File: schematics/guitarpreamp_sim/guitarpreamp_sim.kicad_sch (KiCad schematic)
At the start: 14 parts, among them U1 OPAMP, U2 OPAMP

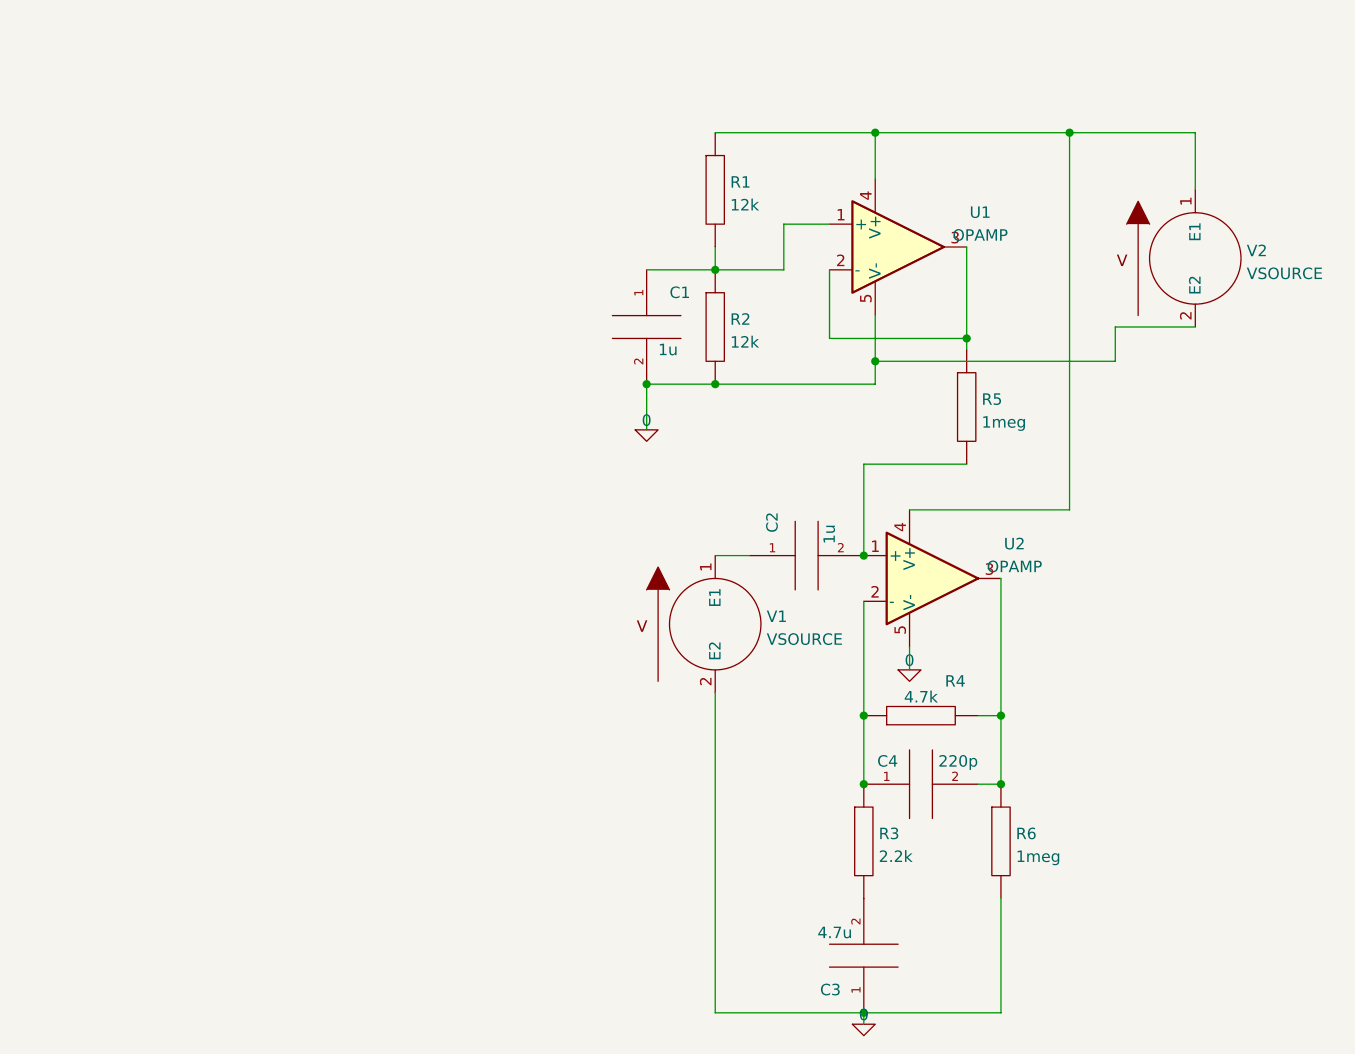
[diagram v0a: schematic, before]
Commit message: pcb: layout changes, c headers: documentation
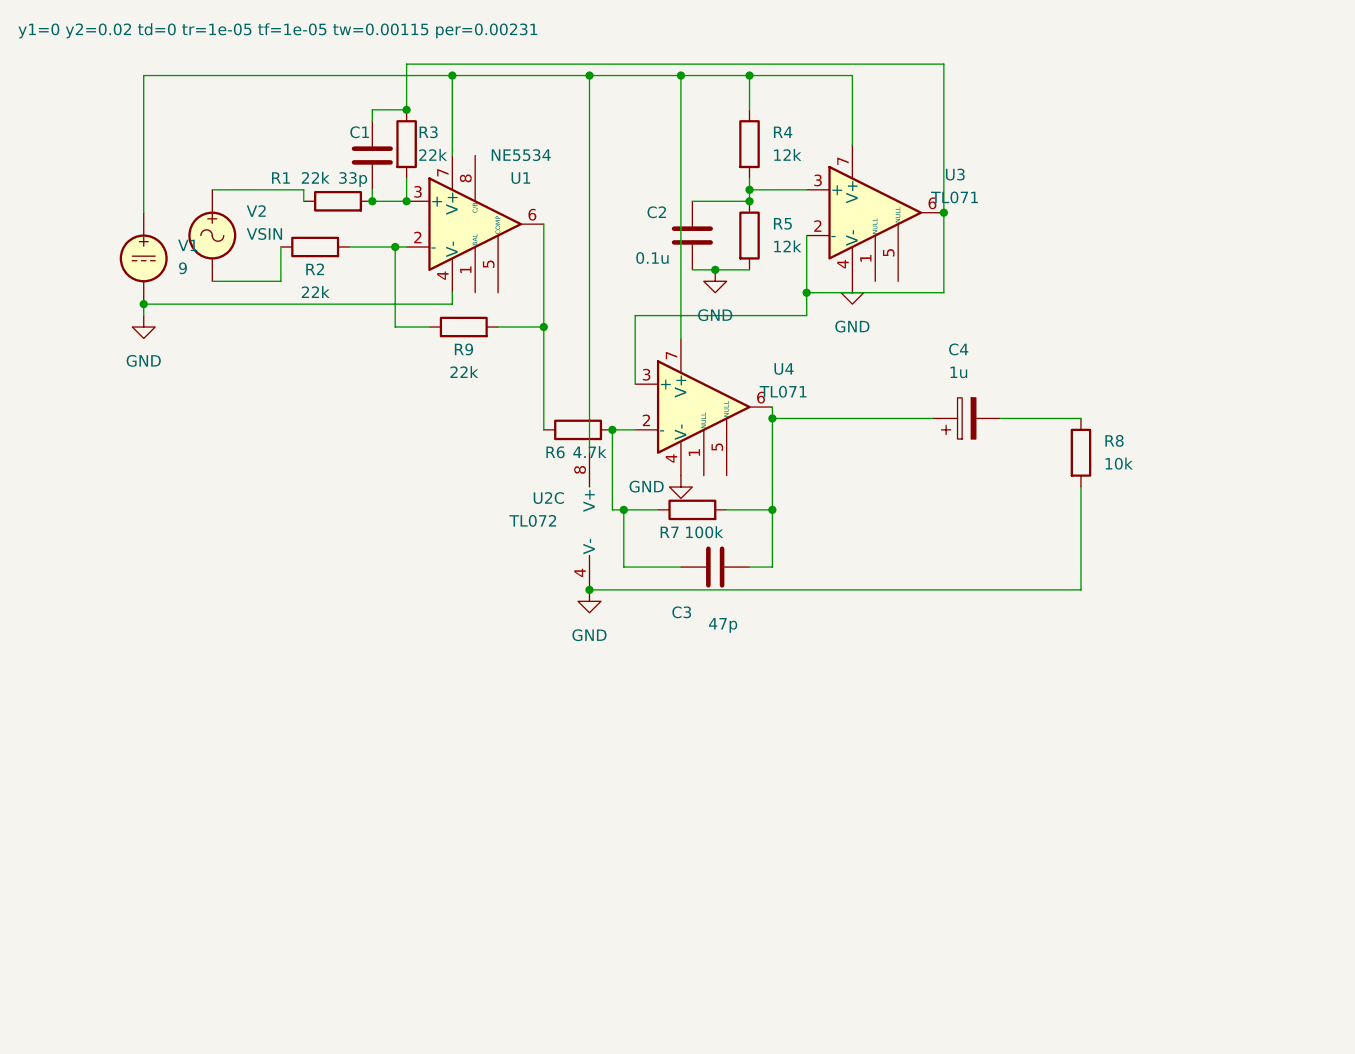
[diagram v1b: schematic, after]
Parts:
- removed C1, C2: 1u, symbol pspice:C
- removed C3: 4.7u, symbol pspice:C
- removed C4: 220p, symbol pspice:C
- removed R1, R2: 12k, symbol pspice:R
- removed R3: 2.2k, symbol pspice:R
- removed R4: 4.7k, symbol pspice:R
- removed R5, R6: 1meg, symbol pspice:R
- removed U1, U2: OPAMP, symbol Simulation_SPICE:OPAMP
- removed V1, V2: VSOURCE, symbol pspice:VSOURCE
- added C1: 33p, symbol Device:C
- added C2: 0.1u, symbol Device:C
- added C3: 47p, symbol Device:C
- added C4: 1u, symbol Device:C_Polarized
- added R1, R2, R3, R9: 22k, symbol Device:R
- added R4, R5: 12k, symbol Device:R
- added R6: 4.7k, symbol Device:R
- added R7: 100k, symbol Device:R
- added R8: 10k, symbol Device:R
- added U1: NE5534, symbol Amplifier_Operational:NE5534
- added U2: TL072, symbol Amplifier_Operational:TL072
- added U3, U4: TL071, symbol Amplifier_Operational:TL071
- added V1: 9, symbol Simulation_SPICE:VDC
- added V2: VSIN, symbol Simulation_SPICE:VSIN
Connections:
- new net: R1.1, V2.1
- new net: C1.2, R1.2, R3.2, U1.3 (+)
- new net: C1.1, R3.1, U3.2 (-), U3.6, U4.3 (+)
- new net: C2.1, R4.2, R5.1, U3.3 (+)
- new net: R2.2, R9.1, U1.2 (-)
- new net: R6.1, R9.2, U1.6
- new net: C3.1, R6.2, R7.1, U4.2 (-)
- new net: C3.2, C4.1, R7.2, U4.6
- new net: R4.1, U1.7 (V+), U2.8 (V+), U3.7 (V+), U4.7 (V+), V1.1
- new net: R2.1, V2.2
- new net: C4.2, R8.1
- new net GND: C2.2, R5.2, R8.2, U1.4 (V-), U2.4 (V-), U3.4 (V-), U4.4 (V-), V1.2
